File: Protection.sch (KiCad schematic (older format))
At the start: 0 parts

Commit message: completion of the layout, initial layout of the protection circuit, reducing number of circuit to 7
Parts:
- added C1, C57: 330p, gatedrive:C_Disc, symbol C
- added D1: ZENER, Diodes_ThroughHole:Diode_DO-41_SOD81_Horizontal_RM10, symbol ZENER
- added IC1: uA741_RevA_14Sep2012, Housings_DIP:DIP-8_W7.62mm_LongPads, symbol uA741_RevA_14Sep2012
- added P18: FromShuntResistor, Terminal_Blocks:TerminalBlock_Pheonix_MKDS1.5-2pol, symbol CONN_01X02
- added P2: FromNtc, Terminal_Blocks:TerminalBlock_Pheonix_MKDS1.5-2pol, symbol CONN_01X02
- added R1: 2.2MEG, Resistors_ThroughHole:Resistor_Horizontal_RM10mm, symbol R
- added R2: 560, Resistors_ThroughHole:Resistor_Horizontal_RM10mm, symbol R
- added R3: 10K, Resistors_ThroughHole:Resistor_Horizontal_RM10mm, symbol R
- added R4, R52, R53, R55, R56, R57, R58: 1.24k, Resistors_ThroughHole:Resistor_Horizontal_RM10mm, symbol R
- added R54: 20k, Resistors_ThroughHole:Resistor_Horizontal_RM10mm, symbol R
- added RV1: POT, Potentiometers:Potentiometer_Bourns_3296W_3-8Zoll_Inline_ScrewUp, symbol POT
- added U2: LM393, Housings_DIP:DIP-14_W7.62mm_LongPads, symbol LM393
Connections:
- new net: C57.2, P18.1 (P1), R53.1, R56.2
- new net: P18.2 (P2), R52.2
- new net: C1.2, C57.1, IC1.3 (+Inp), R52.1, R54.2, R55.1, R56.1
- new net: IC1.2 (-Inp), R53.2, R54.1
- new net: C1.1, IC1.6 (Out), R55.2, R57.1
- new net: R57.2, U2.2 (_)
- new net: RV1.2, U2.3 (+)
- new net: D1.1 (K), R1.1, R2.2, RV1.3, U2.5 (+)
- new net: P2.1 (P1), R3.1, U2.6 (_)
- new net GND1: D1.2 (A), R3.2, RV1.1, U2.8 (V+), U2.8 (V+)
- new net MICSUPP: P2.2 (P2), R2.1, R4.1, R58.1, U2.4 (V-), U2.4 (V-)
- new net ~FAULT: R58.2, U2.1
- new net ~OVERTEMP: R1.2, R4.2, U2.7

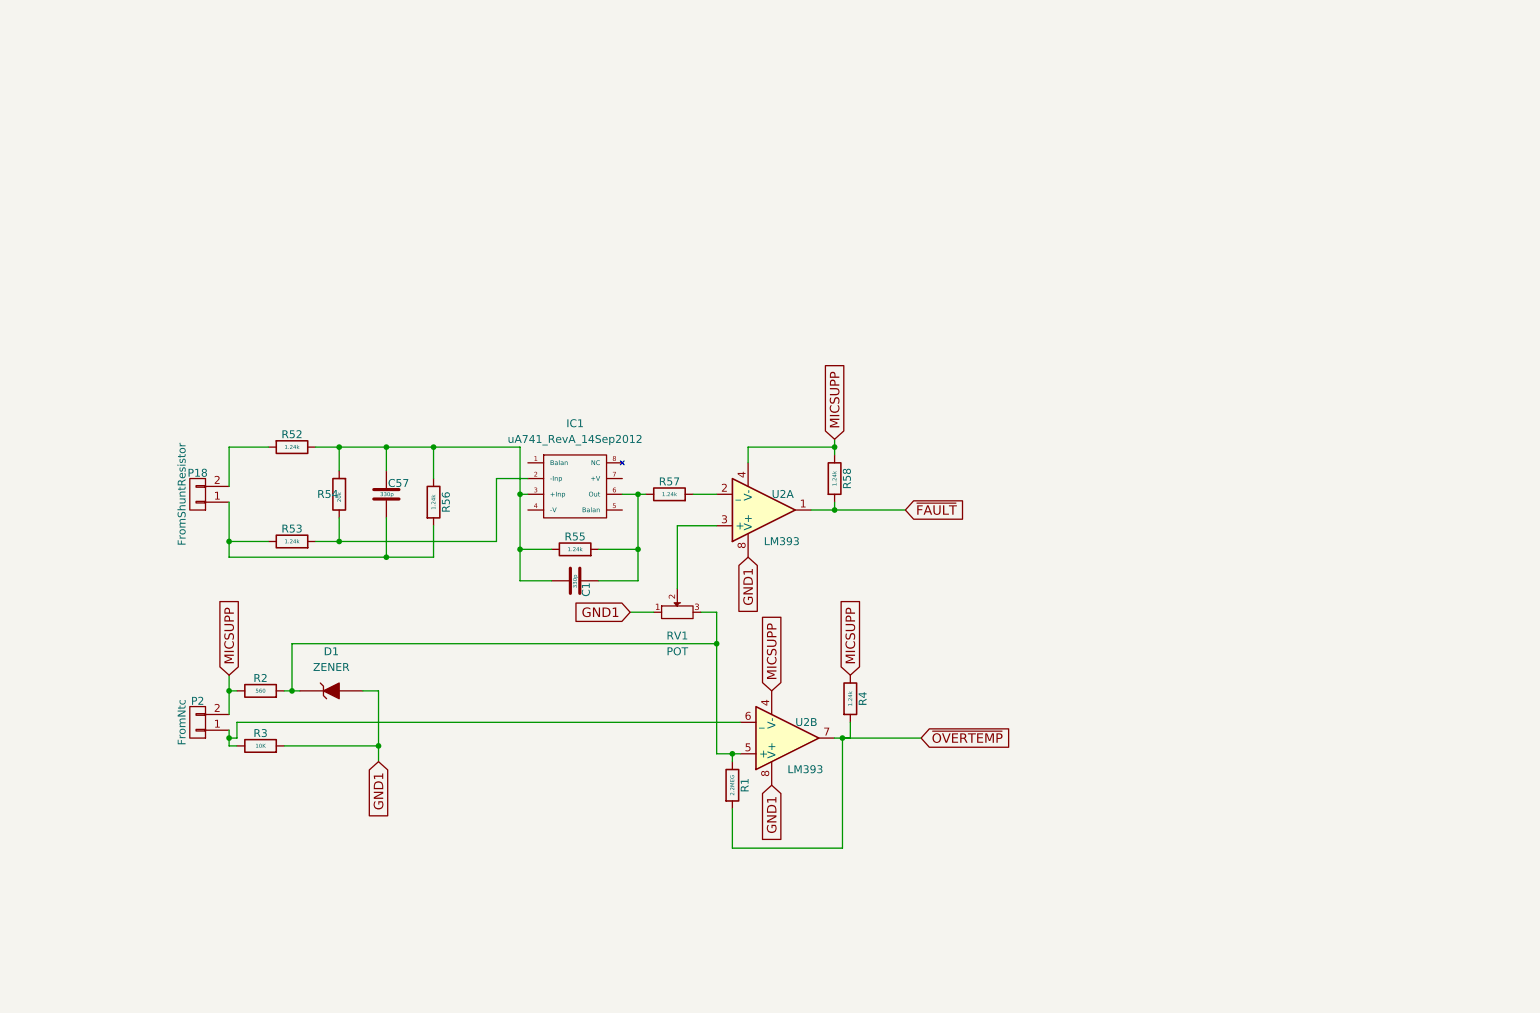
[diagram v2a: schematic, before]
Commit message: yet another enhancements .
the protection section still is incomplete.
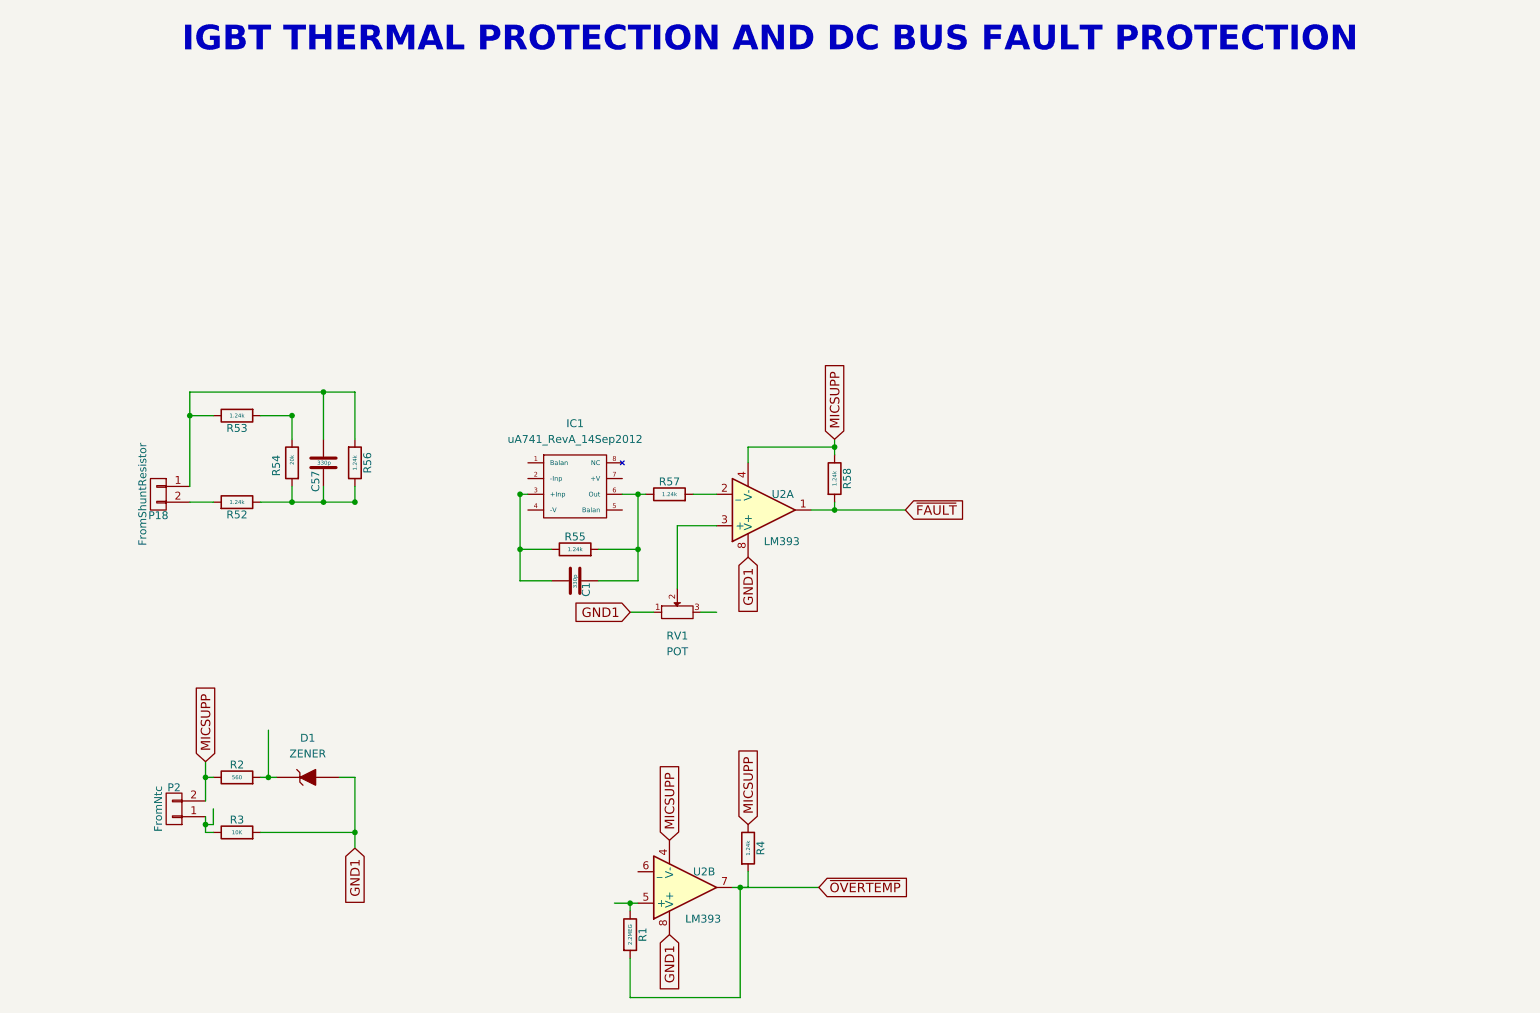
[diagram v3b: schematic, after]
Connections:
- wire segments 55 -> 49
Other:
- note added: "IGBT THERMAL PROTECTION AND DC BUS FAULT PROTECTION"
- moved on the sheet: C57, D1, P18, P2, R1, R2, R3, R4, R52, R53, R54, R56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

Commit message: packup
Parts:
- removed IC1: uA741_RevA_14Sep2012, Housings_DIP:DIP-8_W7.62mm_LongPads, symbol uA741_RevA_14Sep2012
- removed U2: LM393, Housings_DIP:DIP-14_W7.62mm_LongPads, symbol LM393
- added C1: 0.1u, gatedrive:C_Disc, symbol C_Small
- added U802: LM339, Housings_DIP:DIP-14_W7.62mm_LongPads, symbol LM339
- C801: renamed from C57; value 330p -> 33pf; symbol C -> C_Small
- C802: renamed from C1; value 330p -> 33p; symbol C -> C_Small
- R801: renamed from R53; symbol R -> R_Small
- R802: renamed from R52; symbol R -> R_Small
- R803: renamed from R54; symbol R -> R_Small
- R804: renamed from R56; value 1.24k -> 61.9k; symbol R -> R_Small
- R805: renamed from R55; value 1.24k -> 61.9k; symbol R -> R_Small
- R806: renamed from R2; symbol R -> R_Small
- R807: renamed from R3; symbol R -> R_Small
- R808: renamed from R57; value 1.24k -> 10k; symbol R -> R_Small
- R809: renamed from R1; symbol R -> R_Small
- R810: renamed from R58; value 1.24k -> 10k; symbol R -> R_Small
- R811: renamed from R4; symbol R -> R_Small
- RV801: renamed from RV1; value POT -> 10k
- renumbered D1 to D801, P18 to P801, P2 to P802
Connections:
- net labels added: +5V, +ve, -ve, GND
- net labels removed: GND1, MICSUPP
- wire segments 49 -> 62
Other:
- moved on the sheet: C801, C802, D801, P801, P802, R801, R802, R803, R804, R805, R806, R807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
